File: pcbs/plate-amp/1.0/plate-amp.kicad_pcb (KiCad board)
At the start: 2 copper layers, 65 x 95 mm, 32 parts, among them J1 Conn_01x02_Pin, J2 Conn_01x02_Pin, J3 Conn_01x02_Pin, U1 TPA3255DDV, U3 OPA1602, U4 OPA1602

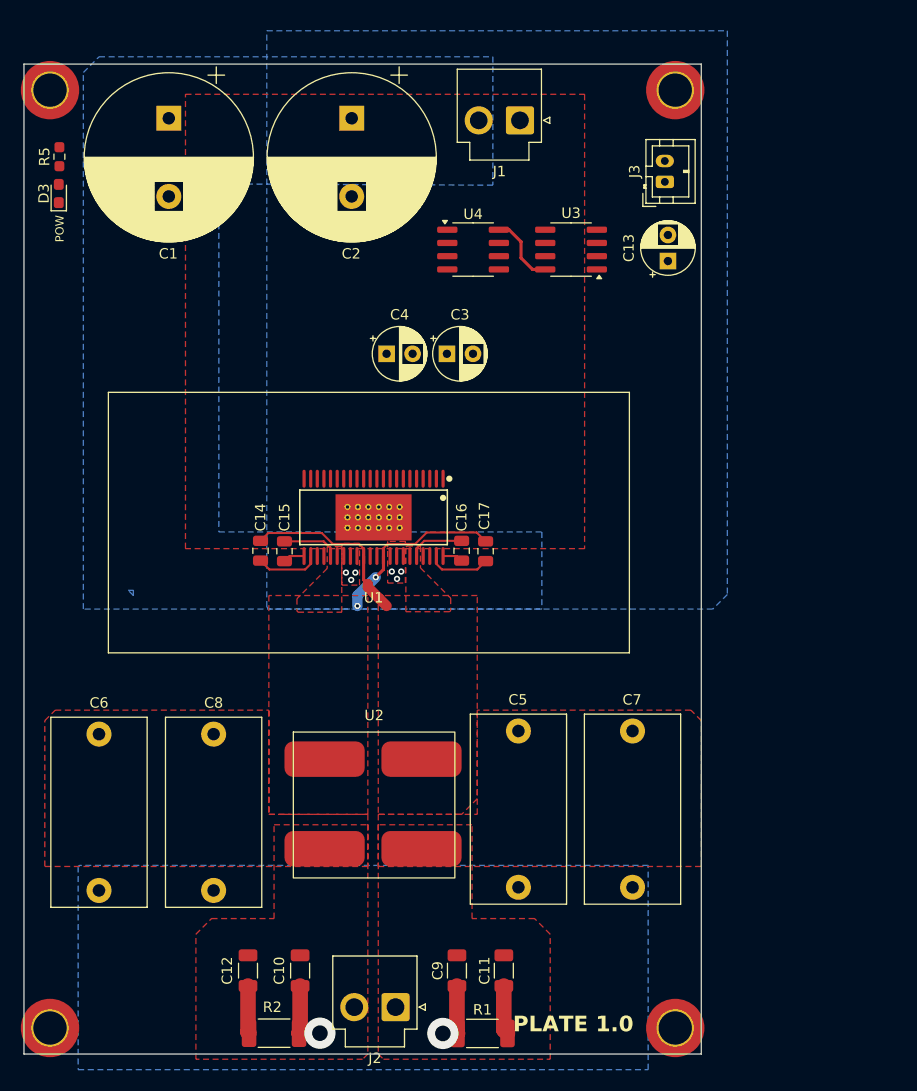
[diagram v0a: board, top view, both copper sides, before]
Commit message: Major updates
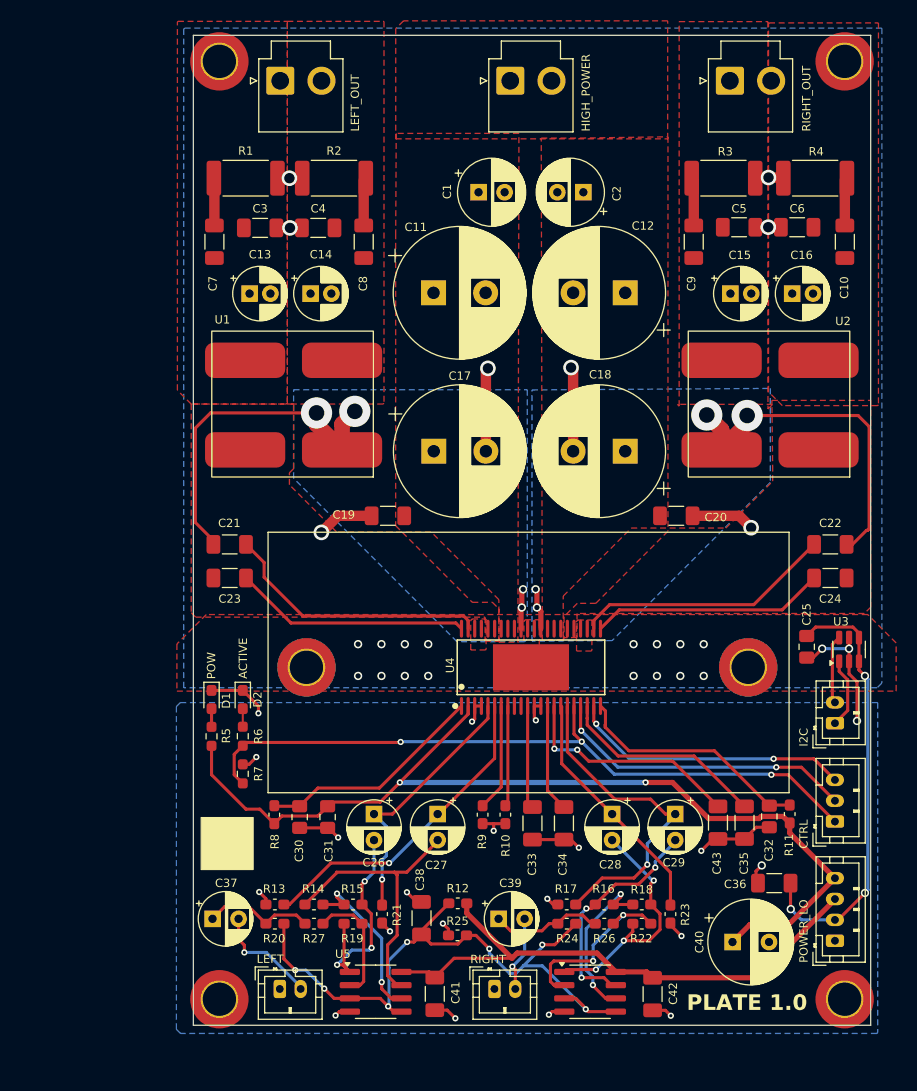
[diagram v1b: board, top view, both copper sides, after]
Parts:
- removed the C17 at (128.2, 107.8)
- added C1: 47U 50V, Capacitor_THT:CP_Radial_D6.3mm_P2.50mm, F.Cu at (127.5, 73.3)
- added C13: 1u 50V, Capacitor_THT:CP_Radial_D5.0mm_P2.00mm, F.Cu at (105.5, 83.0)
- added C18: 1000U 50V, Capacitor_THT:CP_Radial_D12.5mm_P5.00mm, F.Cu at (141.6, 98.2)
- added C19: 1U X7R 50V, Capacitor_SMD:C_1206_3216Metric_Pad1.33x1.80mm_HandSolder, F.Cu at (118.8, 104.3)
- added C20: 1U X7R 50V, Capacitor_SMD:C_1206_3216Metric_Pad1.33x1.80mm_HandSolder, F.Cu at (146.5, 104.3)
- added C21: 33n 100V, Capacitor_SMD:C_1206_3216Metric_Pad1.33x1.80mm_HandSolder, F.Cu at (103.6, 107.1)
- added C22: 33n 100V, Capacitor_SMD:C_1206_3216Metric_Pad1.33x1.80mm_HandSolder, F.Cu at (161.3, 107.1)
- added C23: 33n 100V, Capacitor_SMD:C_1206_3216Metric_Pad1.33x1.80mm_HandSolder, F.Cu at (103.6, 110.3)
- added C24: 33n 100V, Capacitor_SMD:C_1206_3216Metric_Pad1.33x1.80mm_HandSolder, F.Cu at (161.3, 110.3)
- added C25: 0.1u, Capacitor_SMD:C_0805_2012Metric_Pad1.18x1.45mm_HandSolder, F.Cu at (159.0, 116.9)
- added C26: 10u Nichicon 25V, Capacitor_THT:CP_Radial_D5.0mm_P2.50mm, F.Cu at (117.5, 133.0)
- added C27: 10u Nichicon 25V, Capacitor_THT:CP_Radial_D5.0mm_P2.50mm, F.Cu at (123.6, 133.0)
- added C28: 10u Nichicon 25V, Capacitor_THT:CP_Radial_D5.0mm_P2.50mm, F.Cu at (140.3, 133.0)
- added C29: 10u Nichicon 25V, Capacitor_THT:CP_Radial_D5.0mm_P2.50mm, F.Cu at (146.4, 133.0)
- added C30: 0.1u, Capacitor_SMD:C_0805_2012Metric_Pad1.18x1.45mm_HandSolder, F.Cu at (110.4, 133.3)
- added C31: 0.1u, Capacitor_SMD:C_0805_2012Metric_Pad1.18x1.45mm_HandSolder, F.Cu at (113.0, 133.3)
- added C32: 0.1u, Capacitor_SMD:C_0805_2012Metric_Pad1.18x1.45mm_HandSolder, F.Cu at (155.4, 133.2)
- added C33: 1u, Capacitor_SMD:C_1206_3216Metric_Pad1.33x1.80mm_HandSolder, F.Cu at (132.7, 133.9)
- added C34: 1u, Capacitor_SMD:C_1206_3216Metric_Pad1.33x1.80mm_HandSolder, F.Cu at (135.7, 133.9)
- added C35: 1u, Capacitor_SMD:C_1206_3216Metric_Pad1.33x1.80mm_HandSolder, F.Cu at (153.0, 133.8)
- added C36: 10u 50V, Capacitor_SMD:C_1206_3216Metric_Pad1.33x1.80mm_HandSolder, F.Cu at (155.9, 139.6)
- added C38: 47u, Capacitor_SMD:C_1206_3216Metric_Pad1.33x1.80mm_HandSolder, F.Cu at (122.0, 143.0)
- added C39: 10u Nichicon 25V, Capacitor_THT:CP_Radial_D5.0mm_P2.50mm, F.Cu at (129.4, 143.0)
- added C40: 470u 16V, Capacitor_THT:CP_Radial_D8.0mm_P3.50mm, F.Cu at (151.9, 145.2)
- added C41: 10u 50V, Capacitor_SMD:C_1206_3216Metric_Pad1.33x1.80mm_HandSolder, F.Cu at (123.3, 150.2)
- added C42: 10u 50V, Capacitor_SMD:C_1206_3216Metric_Pad1.33x1.80mm_HandSolder, F.Cu at (144.2, 150.2)
- added C43: 47u, Capacitor_SMD:C_1206_3216Metric_Pad1.33x1.80mm_HandSolder, F.Cu at (150.5, 133.8)
- added D2: RED, LED_SMD:LED_0603_1608Metric_Pad1.05x0.95mm_HandSolder, F.Cu at (104.9, 122.0)
- added H3: MountingHole_Pad, MountingHole:MountingHole_3.2mm_M3_DIN965_Pad_TopBottom, F.Cu at (111.0, 118.9)
- added H4: MountingHole_Pad, MountingHole:MountingHole_3.2mm_M3_DIN965_Pad_TopBottom, F.Cu at (153.4, 118.9)
- added J3: Conn_01x02_Pin, Connector_JST:JST_VH_B2P-VH-B_1x02_P3.96mm_Vertical, F.Cu at (151.6, 62.6)
- added J4: Conn_01x02_Pin, Connector_JST:JST_PH_B2B-PH-K_1x02_P2.00mm_Vertical, F.Cu at (161.7, 124.3)
- added J5: Conn_01x03_Pin, Connector_JST:JST_PH_B3B-PH-K_1x03_P2.00mm_Vertical, F.Cu at (161.7, 133.7)
- added J6: Conn_01x04_Pin, Connector_JST:JST_PH_B4B-PH-K_1x04_P2.00mm_Vertical, F.Cu at (161.7, 145.1)
- added J8: Conn_01x02_Pin, Connector_JST:JST_PH_B2B-PH-K_1x02_P2.00mm_Vertical, F.Cu at (129.1, 149.8)
- added R10: 30k, Capacitor_SMD:C_0603_1608Metric_Pad1.08x0.95mm_HandSolder, F.Cu at (130.1, 133.0)
- added R11: 3R3, Capacitor_SMD:C_0603_1608Metric_Pad1.08x0.95mm_HandSolder, F.Cu at (157.4, 133.0)
- added R12: 10k, Capacitor_SMD:C_0603_1608Metric_Pad1.08x0.95mm_HandSolder, F.Cu at (125.5, 141.5)
- added R13: 20k, Capacitor_SMD:C_0603_1608Metric_Pad1.08x0.95mm_HandSolder, F.Cu at (108.0, 141.6)
- added R14: 10k, Capacitor_SMD:C_0603_1608Metric_Pad1.08x0.95mm_HandSolder, F.Cu at (111.7, 141.6)
- added R15: 10k, Capacitor_SMD:C_0603_1608Metric_Pad1.08x0.95mm_HandSolder, F.Cu at (115.5, 141.6)
- added R16: 10k, Capacitor_SMD:C_0603_1608Metric_Pad1.08x0.95mm_HandSolder, F.Cu at (139.6, 141.6)
- added R17: 20k, Capacitor_SMD:C_0603_1608Metric_Pad1.08x0.95mm_HandSolder, F.Cu at (136.0, 141.6)
- added R18: 10k, Capacitor_SMD:C_0603_1608Metric_Pad1.08x0.95mm_HandSolder, F.Cu at (143.2, 141.6)
- added R19: 13k, Capacitor_SMD:C_0603_1608Metric_Pad1.08x0.95mm_HandSolder, F.Cu at (115.5, 143.5)
- added R20: 20k, Capacitor_SMD:C_0603_1608Metric_Pad1.08x0.95mm_HandSolder, F.Cu at (108.0, 143.5)
- added R21: 20k, Capacitor_SMD:C_0603_1608Metric_Pad1.08x0.95mm_HandSolder, F.Cu at (118.3, 142.6)
- added R22: 13k, Capacitor_SMD:C_0603_1608Metric_Pad1.08x0.95mm_HandSolder, F.Cu at (143.2, 143.5)
- added R23: 20k, Capacitor_SMD:C_0603_1608Metric_Pad1.08x0.95mm_HandSolder, F.Cu at (145.9, 142.6)
- added R24: 20k, Capacitor_SMD:C_0603_1608Metric_Pad1.08x0.95mm_HandSolder, F.Cu at (136.0, 143.5)
- added R25: 10k, Capacitor_SMD:C_0603_1608Metric_Pad1.08x0.95mm_HandSolder, F.Cu at (125.5, 144.6)
- added R26: 10k, Capacitor_SMD:C_0603_1608Metric_Pad1.08x0.95mm_HandSolder, F.Cu at (139.6, 143.5)
- added R27: 10k, Capacitor_SMD:C_0603_1608Metric_Pad1.08x0.95mm_HandSolder, F.Cu at (111.7, 143.5)
- added R3: 3R3, Resistor_SMD:R_2512_6332Metric_Pad1.40x3.35mm_HandSolder, F.Cu at (151.0, 72.0)
- added R4: 3R3, Resistor_SMD:R_2512_6332Metric_Pad1.40x3.35mm_HandSolder, F.Cu at (159.8, 72.0)
- added R6: 330R, Resistor_SMD:R_0603_1608Metric_Pad0.98x0.95mm_HandSolder, F.Cu at (104.9, 125.5)
- added R7: 4.7K, Resistor_SMD:R_0603_1608Metric_Pad0.98x0.95mm_HandSolder, F.Cu at (104.9, 129.1)
- added R8: 3R3, Capacitor_SMD:C_0603_1608Metric_Pad1.08x0.95mm_HandSolder, F.Cu at (107.9, 133.0)
- added R9: 22k, Capacitor_SMD:C_0603_1608Metric_Pad1.08x0.95mm_HandSolder, F.Cu at (127.9, 133.0)
- added U2: ~, Custom:UA8014-AL, F.Cu at (155.5, 93.7)
- added U3: TMP100, Package_TO_SOT_SMD:SOT-23-6, F.Cu at (163.1, 117.2)
- C10, C9: value 1n C0G -> 10n 50V C0G; footprint Capacitor_SMD:C_1206_3216Metric -> Capacitor_SMD:C_1206_3216Metric_Pad1.33x1.80mm_HandSolder
- C11, C12: value 10n C0G -> 1000U 50V; footprint Capacitor_SMD:C_1206_3216Metric -> Capacitor_THT:CP_Radial_D12.5mm_P5.00mm
- C14, C15, C16: value 33n C0G -> 1u 50V; footprint Capacitor_SMD:C_0805_2012Metric -> Capacitor_THT:CP_Radial_D5.0mm_P2.00mm
- C17: renamed from C1; value 1000u 63V -> 1000U 50V; footprint Capacitor_THT:CP_Radial_D16.0mm_P7.50mm -> Capacitor_THT:CP_Radial_D12.5mm_P5.00mm
- C2: value 1000u 63V -> 47U 50V; footprint Capacitor_THT:CP_Radial_D16.0mm_P7.50mm -> Capacitor_THT:CP_Radial_D6.3mm_P2.50mm
- C3, C4: value 10u Nichicon 25V -> 1n 50V C0G; footprint Capacitor_THT:CP_Radial_D5.0mm_P2.50mm -> Capacitor_SMD:C_1206_3216Metric_Pad1.33x1.80mm_HandSolder
- C5, C6: value 470n 100V -> 1n 50V C0G; footprint Capacitor_THT:C_Rect_L18.0mm_W9.0mm_P15.00mm_FKS3_FKP3 -> Capacitor_SMD:C_1206_3216Metric_Pad1.33x1.80mm_HandSolder
- C7, C8: value 470n 100V -> 10n 50V C0G; footprint Capacitor_THT:C_Rect_L18.0mm_W9.0mm_P15.00mm_FKS3_FKP3 -> Capacitor_SMD:C_1206_3216Metric_Pad1.33x1.80mm_HandSolder
- R1, R2: footprint Resistor_SMD:R_2010_5025Metric_Pad1.40x2.65mm_HandSolder -> Resistor_SMD:R_2512_6332Metric_Pad1.40x3.35mm_HandSolder
- R5: value 150R -> 3K
- moved H2 120.1 mm to (162.7, 60.7), turned to -90 degrees
- moved H6 115.9 mm to (162.7, 150.7), turned to -90 degrees
- moved H1 102.6 mm to (102.7, 60.7), turned to -90 degrees
- moved H5 97.6 mm to (102.7, 150.7), turned to -90 degrees
- moved J1 89.6 mm to (108.5, 62.6), turned to 0 degrees
- moved C10 87.3 mm to (162.7, 78.0)
- moved J7 85.8 mm to (108.5, 149.8), turned to 0 degrees
- moved R1 85.2 mm to (105.2, 72.0)
- moved C6 82.8 mm to (158.1, 76.7), turned to 0 degrees
- moved R2 82.3 mm to (113.7, 72.0)
- moved C37 76.8 mm to (102.0, 143.0), turned to 0 degrees
- moved C12 74.4 mm to (141.6, 83.0), turned to 180 degrees
- moved C7 73.8 mm to (102.2, 78.0)
- moved U5 73.7 mm to (117.7, 150.0), turned to 0 degrees
- moved C9 73.5 mm to (148.2, 78.0)
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- renumbered C13 to C37, D3 to D1, H4 to H1, H3 to H2, H2 to H5, H1 to H6, J2 to J1, J1 to J2, J3 to J7, U2 to U1, U1 to U4, U3 to U5, U4 to U6
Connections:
- net AUDIO_IN renamed LEFT_IN
- C10 pad 1: SPEAKER_OUT2 -> Net-(C10-Pad1)
- C10 pad 2: MID -> SPEAKERR_NEG
- C11 pad 1: Net-(C11-Pad1) -> 48V
- C11 pad 2: SPEAKER_OUT1 -> PGND
- C12 pad 1: SPEAKER_OUT2 -> 48V
- C12 pad 2: Net-(C12-Pad2) -> PGND
- C14 pad 1: OUT1 -> PGND
- C14 pad 2: Net-(U1-BST_C) -> SPEAKERL_NEG
- C15 pad 1: OUT2 -> SPEAKERR_POS
- C15 pad 2: Net-(U1-BST_D) -> PGND
- C16 pad 1: OUT1 -> PGND
- C16 pad 2: Net-(U1-BST_A) -> SPEAKERR_NEG
- C17 pad 2: GND -> PGND
- C2 pad 2: GND -> PGND
- C3 pad 1: INA -> SPEAKERL_POS
- C3 pad 2: Net-(U1-INPUT_A) -> PGND
- C37 pad 1: Net-(U3A-+) -> Net-(C37-Pad1)
- C4 pad 1: INB -> PGND
- C4 pad 2: Net-(U1-INPUT_B) -> SPEAKERL_NEG
- C5 pad 1: MID -> SPEAKERR_POS
- C5 pad 2: SPEAKER_OUT1 -> PGND
- C6 pad 1: SPEAKER_OUT2 -> PGND
- C6 pad 2: MID -> SPEAKERR_NEG
- C7 pad 1: MID -> SPEAKERL_POS
- C7 pad 2: SPEAKER_OUT1 -> Net-(C7-Pad2)
- C8 pad 1: SPEAKER_OUT2 -> Net-(C8-Pad1)
- C8 pad 2: MID -> SPEAKERL_NEG
- C9 pad 1: MID -> SPEAKERR_POS
- C9 pad 2: SPEAKER_OUT1 -> Net-(C9-Pad2)
- J1 pad 1: SPEAKER_OUT1 -> SPEAKERL_POS
- J1 pad 2: SPEAKER_OUT2 -> SPEAKERL_NEG
- J2 pad 1: GND -> PGND
- R1 pad 1: MID -> Net-(C7-Pad2)
- R1 pad 2: Net-(C11-Pad1) -> PGND
- R2 pad 1: Net-(C12-Pad2) -> PGND
- R2 pad 2: MID -> Net-(C8-Pad1)
- R5 pad 1: 3V3 -> 12V
- U1 pad 1: OUT2 -> OUTB
- U1 pad 2: SPEAKER_OUT2 -> SPEAKERL_NEG
- U1 pad 3: SPEAKER_OUT1 -> SPEAKERL_POS
- U1 pad 4: OUT1 -> OUTA
- U4 pad 1: unconnected-(U1-GVDD_AB-Pad1) -> Net-(U4-GVDD_AB)
- U4 pad 11: unconnected-(U1-DVDD-Pad11) -> Net-(U4-DVDD)
- U4 pad 14: unconnected-(U1-AVDD-Pad14) -> Net-(U4-AVDD)
- U4 pad 15: unconnected-(U1-C_START-Pad15) -> Net-(U4-C_START)
- U4 pad 16: unconnected-(U1-INPUT_C-Pad16) -> RIGHT_A
- U4 pad 17: unconnected-(U1-INPUT_D-Pad17) -> RIGHT_B
- U4 pad 18: unconnected-(U1-~{RESET}-Pad18) -> RESET
- U4 pad 19: unconnected-(U1-~{FAULT}-Pad19) -> FAULT
- U4 pad 2: unconnected-(U1-VDD-Pad2) -> 12V
- U4 pad 20: unconnected-(U1-VBG-Pad20) -> Net-(U4-VBG)
- U4 pad 21: unconnected-(U1-~{CLIP_OTW}-Pad21) -> CLIP
- U4 pad 22: unconnected-(U1-GVDD_CD-Pad22) -> Net-(U4-GVDD_CD)
- U4 pad 23: Net-(U1-BST_D) -> Net-(U4-BST_D)
- U4 pad 24: Net-(U1-BST_C) -> Net-(U4-BST_C)
- U4 pad 25: GND2 -> PGND
- U4 pad 26: GND2 -> PGND
- U4 pad 27: OUT2 -> OUTD
- U4 pad 28: OUT2 -> OUTD
- U4 pad 3: unconnected-(U1-M1-Pad3) -> GND
- U4 pad 32: OUT1 -> OUTC
- U4 pad 33: GNDMID -> PGND
- U4 pad 34: GNDMID -> PGND
- U4 pad 35: OUT2 -> OUTB
- U4 pad 39: OUT1 -> OUTA
- U4 pad 4: unconnected-(U1-M2-Pad4) -> GND
- U4 pad 40: OUT1 -> OUTA
- U4 pad 41: GND1 -> PGND
- U4 pad 42: GND1 -> PGND
- U4 pad 44: Net-(U1-BST_A) -> Net-(U4-BST_A)
- U4 pad 45: GND -> PGND
- U4 pad 5: Net-(U1-INPUT_A) -> LEFT_A
- U4 pad 6: Net-(U1-INPUT_B) -> LEFT_B
- U4 pad 7: unconnected-(U1-OC_ADJ-Pad7) -> Net-(U4-OC_ADJ)
- U4 pad 8: unconnected-(U1-FREQ_ADJ-Pad8) -> Net-(U4-FREQ_ADJ)
- U5 pad 1: unconnected-(U3-Pad1) -> Net-(C26-Pad2)
- U5 pad 2: unconnected-(U3A---Pad2) -> Net-(U5A--)
- U5 pad 3: Net-(U3A-+) -> 4.75V
- U5 pad 5: unconnected-(U3B-+-Pad5) -> 4.75V
- U5 pad 6: unconnected-(U3B---Pad6) -> Net-(U5B--)
- U5 pad 7: unconnected-(U3-Pad7) -> Net-(C27-Pad2)
- U5 pad 8: 12V -> 9.5V
- U6 pad 1: unconnected-(U4-Pad1) -> Net-(C28-Pad2)
- U6 pad 2: unconnected-(U4A---Pad2) -> Net-(U6A--)
- U6 pad 3: unconnected-(U4A-+-Pad3) -> 4.75V
- U6 pad 5: unconnected-(U4B-+-Pad5) -> 4.75V
- U6 pad 6: unconnected-(U4B---Pad6) -> Net-(U6B--)
- U6 pad 7: unconnected-(U4-Pad7) -> Net-(C29-Pad2)
- U6 pad 8: 12V -> 9.5V
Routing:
- net 12V: track 6.94 -> 92.6 mm, vias 0 -> 2
- net RESET: track 0.00 -> 68.1 mm, vias 0 -> 3
- net 4.75V: track 0.00 -> 60.6 mm, vias 0 -> 7
- net GND: track 0.00 -> 59.7 mm, vias 0 -> 22
- net 9.5V: track 0.00 -> 54.0 mm
- net 3V3: track 0.00 -> 41.4 mm, vias 0 -> 3
- net PGND: track 0.00 -> 37.8 mm, vias 0 -> 24
- net OUTC: track 0.00 -> 36.8 mm, vias 0 -> 4
- net OUTB: track 0.00 -> 36.4 mm, vias 0 -> 4
- net RIGHT_B: track 0.00 -> 31.9 mm, vias 0 -> 1
- net LEFT_B: track 0.00 -> 31.1 mm, vias 0 -> 1
- net FAULT: track 0.00 -> 29.5 mm, vias 0 -> 2
- net Net-(C27-Pad2): track 0.00 -> 27.1 mm
- net CLIP: track 0.00 -> 27.1 mm, vias 0 -> 2
- net LEFT_A: track 0.00 -> 25.3 mm, vias 0 -> 1
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- added copper zone on F.Cu, net OUTA
- added copper zone on B.Cu, net OUTB
- added copper zone on B.Cu, net OUTC
- added copper zone on F.Cu, net OUTD
- added copper zone on B.Cu, net PGND
- added copper zone on F.Cu, net PGND
- added copper zone on F.Cu, net SPEAKERL_NEG
- added copper zone on F.Cu, net SPEAKERL_POS
- added copper zone on F.Cu, net SPEAKERR_NEG
- added copper zone on F.Cu, net SPEAKERR_POS
- removed copper zone on B.Cu, net 48V
- removed copper zone on F.Cu, net GND
- removed copper zone on B.Cu, net MID
- removed copper zone on F.Cu, net OUT1
- removed copper zone on F.Cu, net OUT2
- removed copper zone on F.Cu, net SPEAKER_OUT1
- removed copper zone on F.Cu, net SPEAKER_OUT2
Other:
- board text added: "ACTIVE"
- board text added: "CTRL"
- board text added: "HIGH_POWER"
- board text added: "I2C"
- board text added: "LEFT"
- board text added: "LEFT_OUT"
- board text added: "POWER_LO"
- board text added: "RIGHT"
- board text added: "RIGHT_OUT"
